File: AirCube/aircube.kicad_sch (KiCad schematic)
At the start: 18 parts, among them J1 Conn_01x04, J2 Connector, USB-TYPE-C-16P, U1 ESP32-C6-MINI-1, U2 AMS1117, U3 USBLC6-2SC6

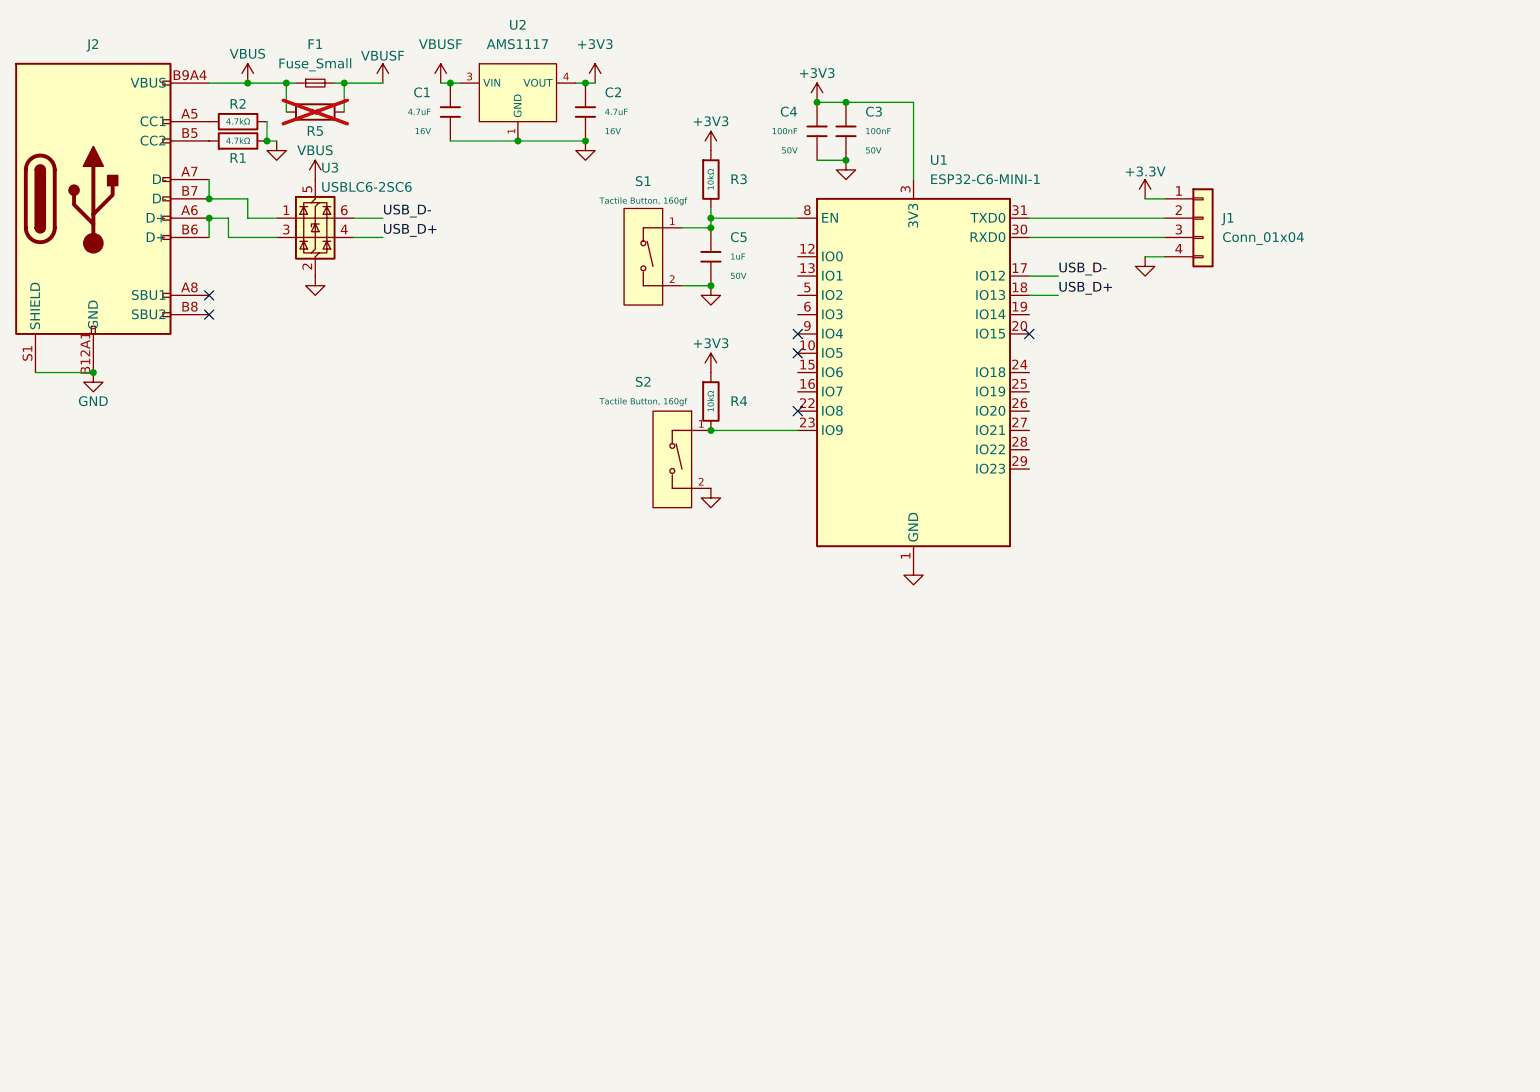
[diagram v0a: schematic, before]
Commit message: wip
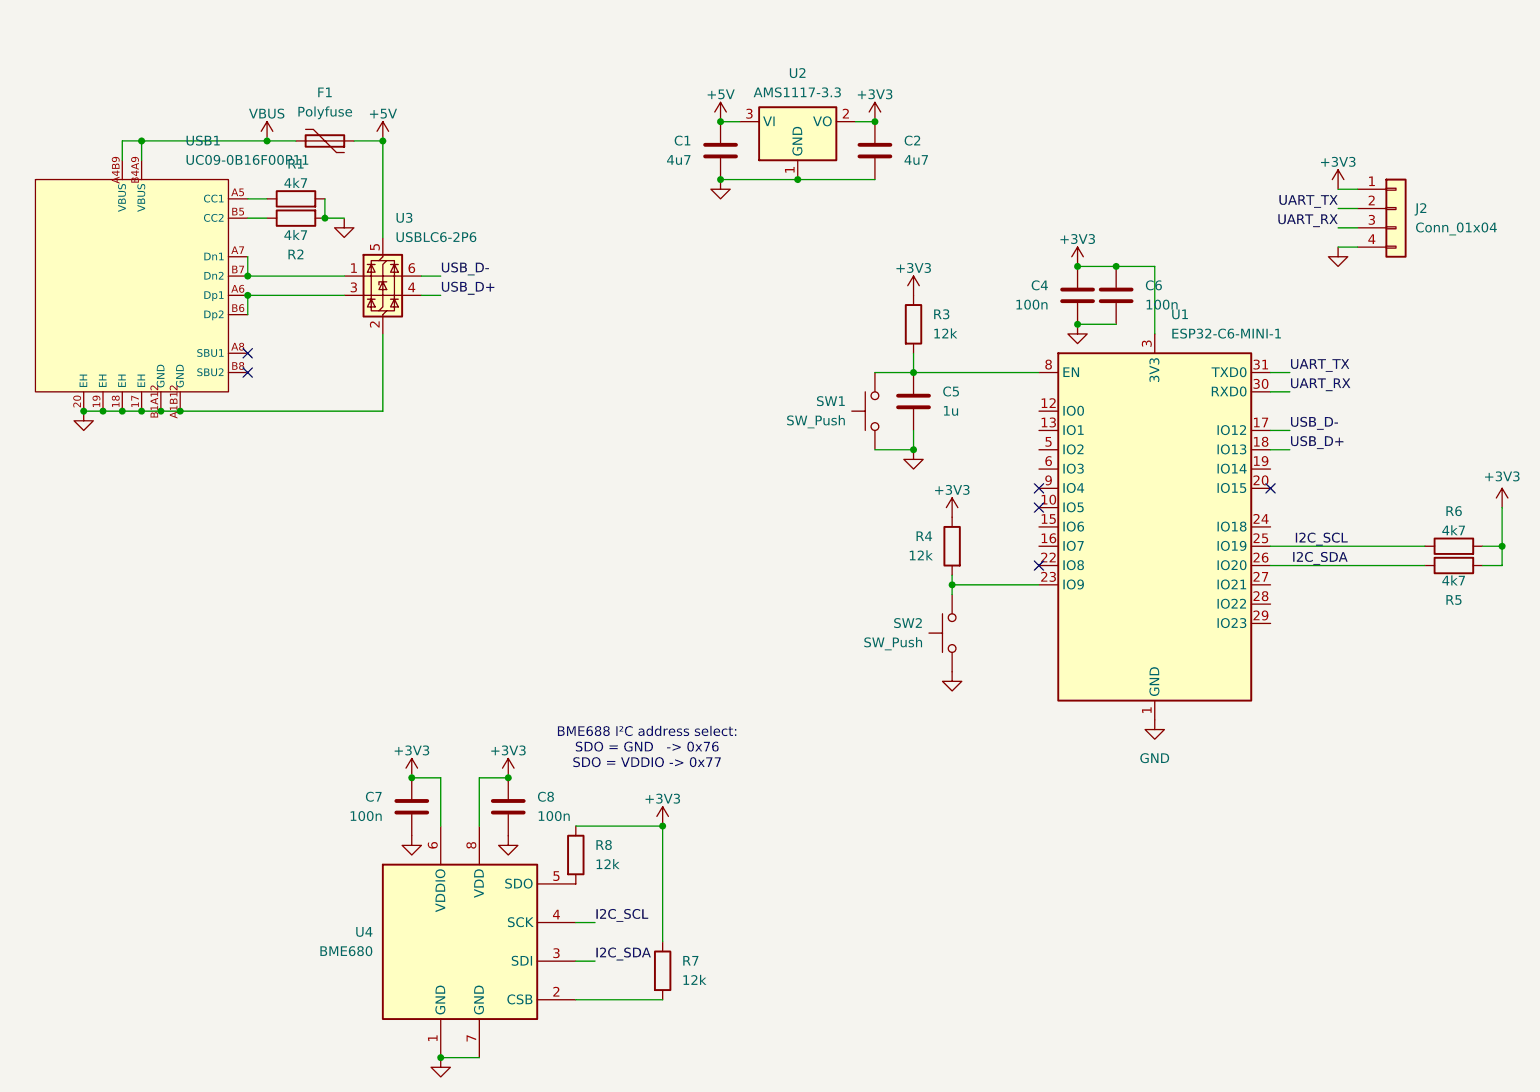
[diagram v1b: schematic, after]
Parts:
- removed C1, C2: 4.7uF, PCM_JLCPCB:C_0603, symbol PCM_JLCPCB-Capacitors:0603,4.7uF
- removed C3, C4: 100nF, PCM_JLCPCB:C_0603, symbol PCM_JLCPCB-Capacitors:0603,100nF
- removed C5: 1uF, PCM_JLCPCB:C_0603, symbol PCM_JLCPCB-Capacitors:0603,1uF
- removed F1: Fuse_Small, Fuse:Fuse_1812_4532Metric_Pad1.30x3.40mm_HandSolder, symbol Device:Fuse_Small
- removed J1: Conn_01x04, Connector_PinHeader_2.54mm:PinHeader_1x04_P2.54mm_Vertical, symbol Connector_Generic:Conn_01x04
- removed J2: Connector, USB-TYPE-C-16P, PCM_JLCPCB:TYPE-C-SMD_HX-TYPE-C-16PIN, symbol PCM_JLCPCB-Extended:Connector, USB-TYPE-C-16P
- removed R1, R2: 4.7kΩ, PCM_JLCPCB:R_0603, symbol PCM_JLCPCB-Resistors:0603,4.7kΩ
- removed R3, R4: 10kΩ, PCM_JLCPCB:R_0603, symbol PCM_JLCPCB-Resistors:0603,10kΩ
- removed R5: 0Ω, PCM_JLCPCB:R_0603, symbol PCM_JLCPCB-Resistors:0603,0Ω
- removed S1, S2: Tactile Button, 160gf, PCM_JLCPCB:SW_TS-1088-AR02016, symbol PCM_JLCPCB-Connectors_Buttons:Tactile Button, 160gf, 12V, 50mA, 4.0mm
- removed U2: AMS1117, PCM_JLCPCB:SOT-223-3_L6.5-W3.4-P2.30-LS7.0-BR, symbol PCM_JLCPCB-Power:LDO, 3.3V, 1A
- removed U3: USBLC6-2SC6, Package_TO_SOT_SMD:SOT-23-6, symbol Power_Protection:USBLC6-2SC6
- added C1, C2: 4u7, Capacitor_SMD:C_0603_1608Metric, symbol Device:C
- added C4, C6, C7, C8: 100n, Capacitor_SMD:C_0603_1608Metric, symbol Device:C
- added C5: 1u, Capacitor_SMD:C_0603_1608Metric, symbol Device:C
- added F1: Polyfuse, Fuse:Fuse_1812_4532Metric, symbol Device:Polyfuse
- added J2: Conn_01x04, Connector_PinHeader_2.54mm:PinHeader_1x04_P2.54mm_Vertical, symbol Connector_Generic:Conn_01x04
- added R1, R2, R5, R6: 4k7, Resistor_SMD:R_0603_1608Metric, symbol Device:R
- added R3, R4, R7, R8: 12k, Resistor_SMD:R_0603_1608Metric, symbol Device:R
- added SW1, SW2: SW_Push, symbol Switch:SW_Push
- added U2: AMS1117-3.3, Package_TO_SOT_SMD:SOT-223-3_TabPin2, symbol Regulator_Linear:AMS1117-3.3
- added U3: USBLC6-2P6, Package_TO_SOT_SMD:SOT-666, symbol Power_Protection:USBLC6-2P6
- added U4: BME680, Package_LGA:Bosch_LGA-8_3x3mm_P0.8mm_ClockwisePinNumbering, symbol Sensor:BME680
- added USB1: UC09-0B16F00P11, lcsc_footprints:C36936538_USB-C_UC09-0B16F00P11, symbol lcsc_imported:UC09-0B16F00P11
- U1: LCSC C5366877 -> (none)
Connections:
- net +3V3: now also C2.1, C4.1, C6.1, C7.1, C8.1, J2.1 (Pin_1), R3.1, R4.1, R5.2, R6.2, R7.1, R8.1, U2.2 (VO), U4.6 (VDDIO), U4.8 (VDD)
- net GND: now also C1.2, C2.2, C4.2, C5.2, C6.2, C7.2, C8.2, J2.4 (Pin_4), R1.2, R2.2, SW1.2, SW2.2, U2.1 (GND), U3.2 (GND), U4.1 (GND), U4.7 (GND), USB1.17 (EH), USB1.18 (EH), USB1.19 (EH), USB1.20 (EH), USB1.A1B12 (GND), USB1.B1A12 (GND)
- net USB_D+: now also U3.4 (I/O2)
- net USB_D-: now also U3.6 (I/O1)
- net VBUS: now also F1.2, USB1.A4B9 (VBUS), USB1.B4A9 (VBUS)
- net at U1.23 (IO9): now also R4.2, SW2.1
- net at U1.8 (EN): now also C5.1, R3.2, SW1.1
- net UART_TX: now reaches U1.31 (TXD0)
- net UART_TX: now also J2.2 (Pin_2)
- net UART_RX: now reaches U1.30 (RXD0)
- net UART_RX: now also J2.3 (Pin_3)
- net I2C_SCL: now reaches U1.25 (IO19)
- net I2C_SCL: now also R6.1, U4.4 (SCK)
- net I2C_SDA: now reaches U1.26 (IO20)
- net I2C_SDA: now also R5.1, U4.3 (SDI)
- new net: R7.2, U4.2 (CSB)
- new net: R8.2, U4.5 (SDO)
- new net: U3.1 (I/O1), USB1.A7 (Dn1), USB1.B7 (Dn2)
- new net: U3.3 (I/O2), USB1.A6 (Dp1), USB1.B6 (Dp2)
- new net: R1.1, USB1.A5 (CC1)
- new net: R2.1, USB1.B5 (CC2)
- new net +5V: C1.1, F1.1, U2.3 (VI), U3.5 (VBUS)
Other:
- note added: "BME688 I²C address select: SDO = GND -> 0x76 SDO = VDDIO -> 0x77"
